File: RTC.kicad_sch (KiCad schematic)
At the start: 12 parts, among them IC7 74LVC1G07QSE-7, J7 Molex 470531000, U1 PCF8563T, U10 EMC2301-1-ACZL-TR, Y2 X32K768S301

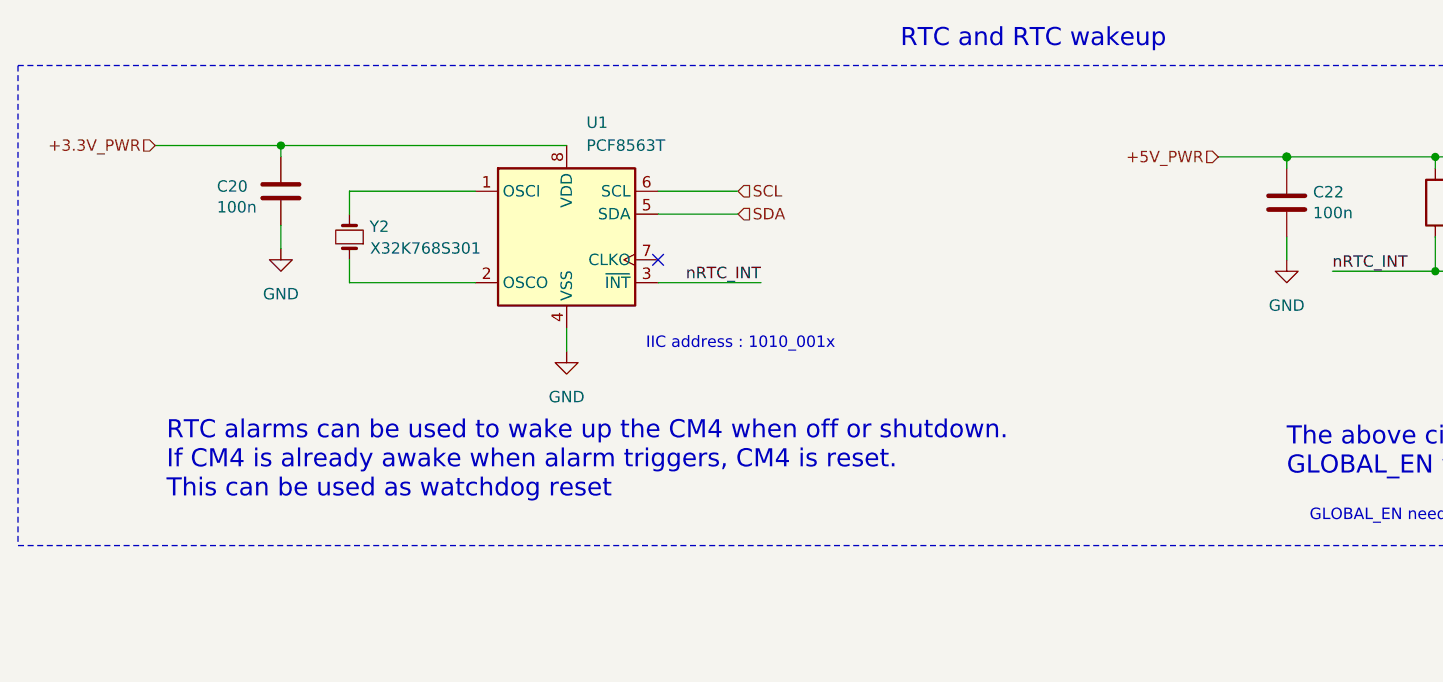
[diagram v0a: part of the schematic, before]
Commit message: small changes for ravi
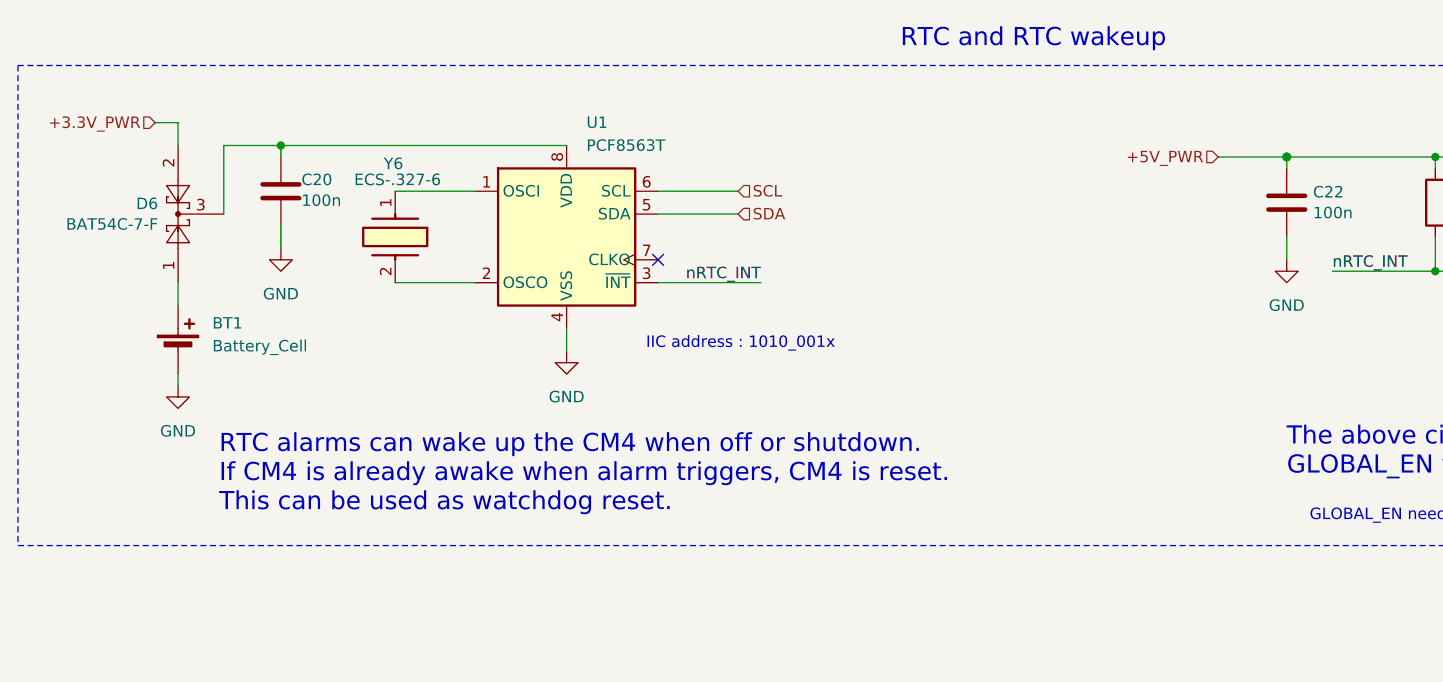
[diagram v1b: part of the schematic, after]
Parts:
- removed Y2: X32K768S301, Crystal:Crystal_SMD_3215-2Pin_3.2x1.5mm, symbol Device:Crystal_Small
- added BT1: Battery_Cell, symbol Device:Battery_Cell
- added D6: BAT54C-7-F, Package_TO_SOT_SMD:SOT-23, symbol Diode:BAT54C
- added Y6: ECS-.327-6, ECS327616RTR, symbol ECS-.327-6-16R-TR:ECS-.327-6-16R-TR
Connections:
- net +3.3V_PWR: now also D6.2; no longer C20.1, U1.8 (VDD)
- net GND: now also BT1.2 (-)
- net at U1.2 (OSCO): now also Y6.2
- net at U1.1 (OSCI): now also Y6.1
- new net: BT1.1 (+), D6.1
- new net: C20.1, D6.3, U1.8 (VDD)
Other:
- note added: "RTC alarms can wake up the CM4 when off or shutdown. If CM4 is already awake when alarm triggers, CM4 is reset. This can be used as watchdog reset."
- note removed: "RTC alarms can be used to wake up the CM4 when off or shutdown. If CM4 is already awake when alarm triggers, CM4 is reset. This can be used as watchdog reset"
